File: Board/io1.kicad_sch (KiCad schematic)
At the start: 1 part, among them U1 XC6SLX9-TQG144

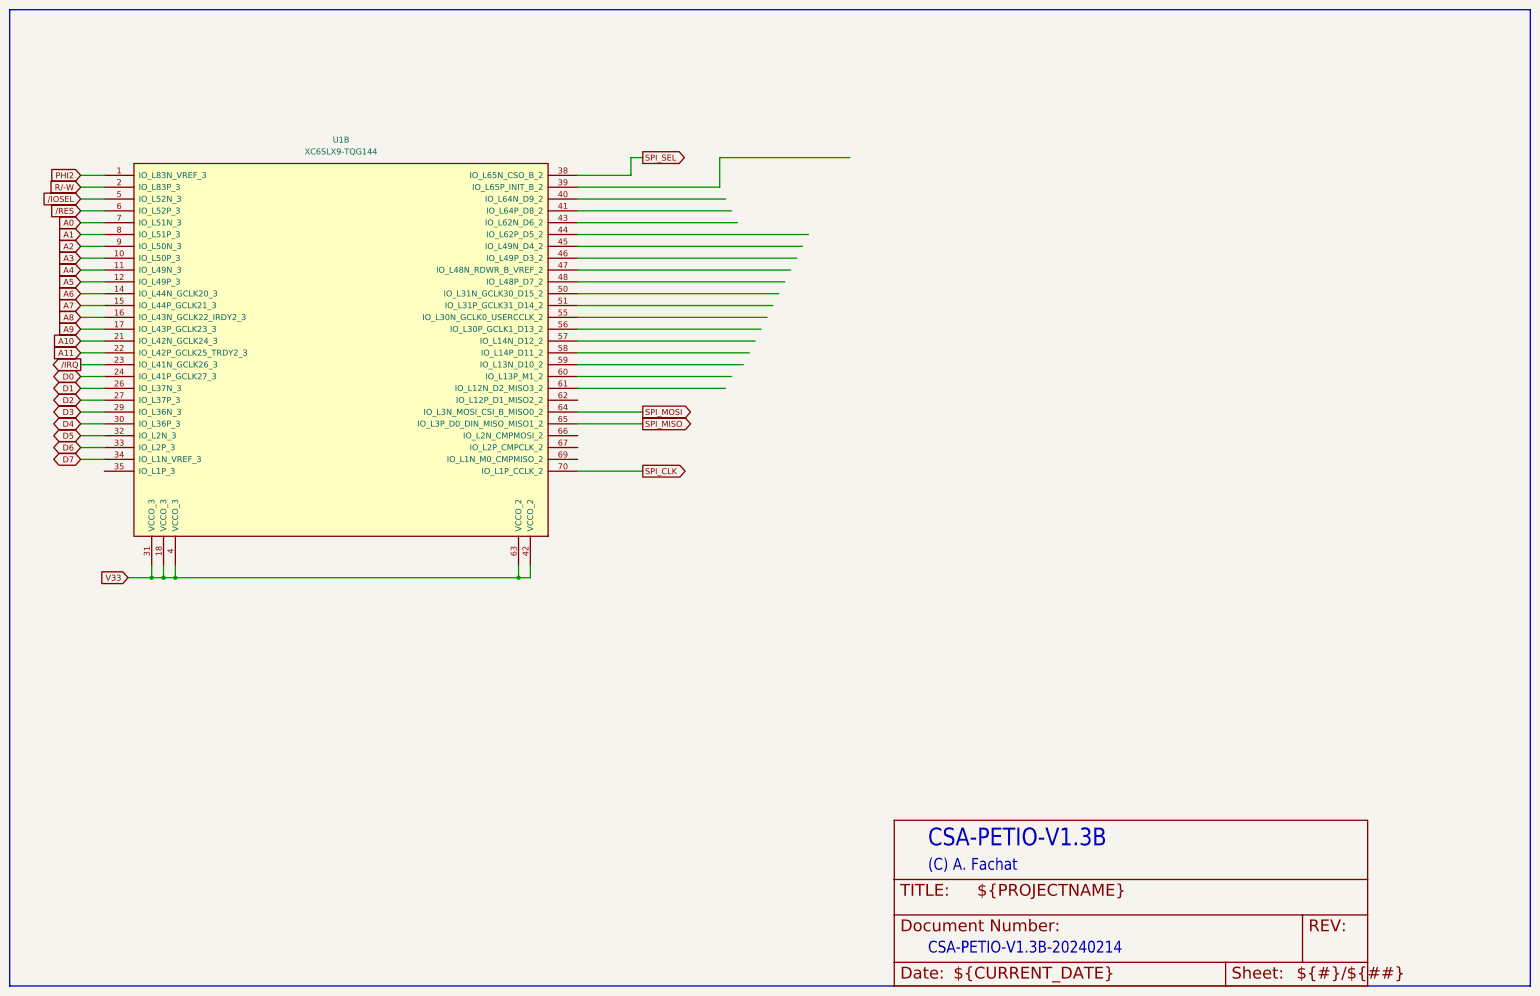
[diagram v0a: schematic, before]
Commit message: update
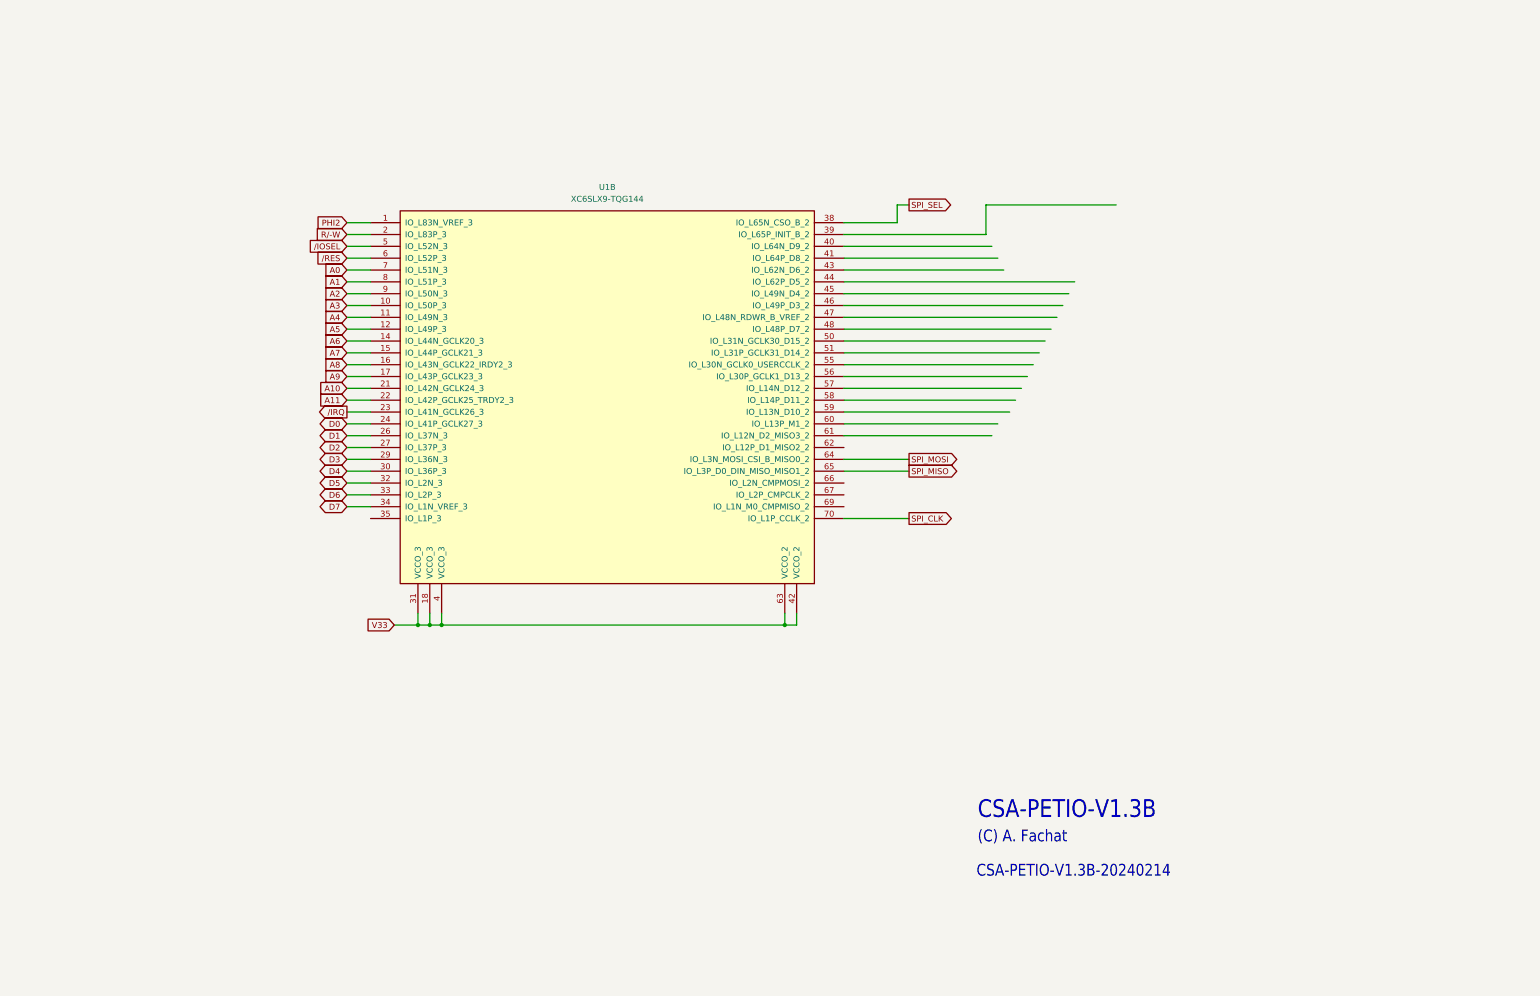
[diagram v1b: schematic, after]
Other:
- moved on the sheet: U1B
